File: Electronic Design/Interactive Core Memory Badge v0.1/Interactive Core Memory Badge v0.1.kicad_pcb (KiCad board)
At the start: 2 copper layers, 8 parts, among them Q1 MMBT4403LT1G, Q2 MMBT4401LT1G, U1 Teensy-LC

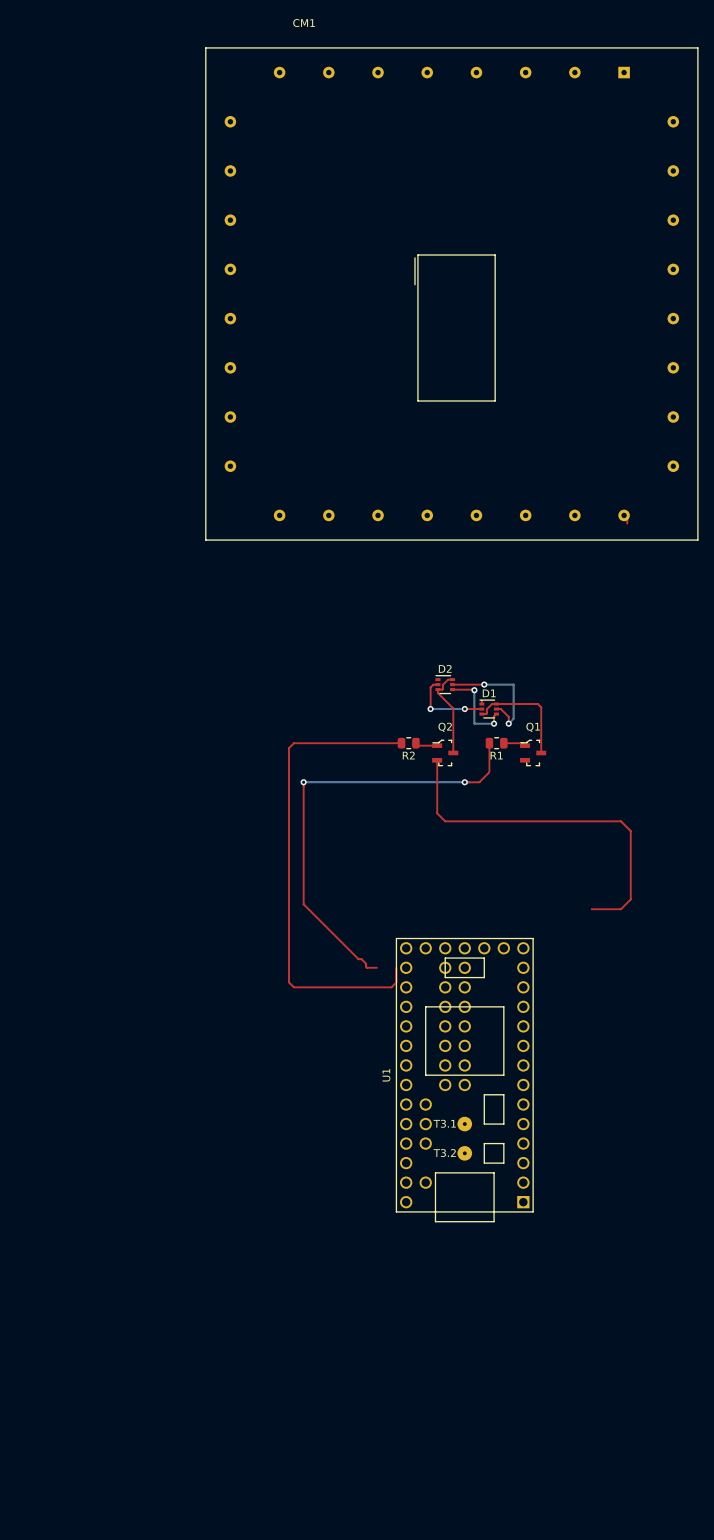
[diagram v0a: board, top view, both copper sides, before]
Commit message: Schematic Complete
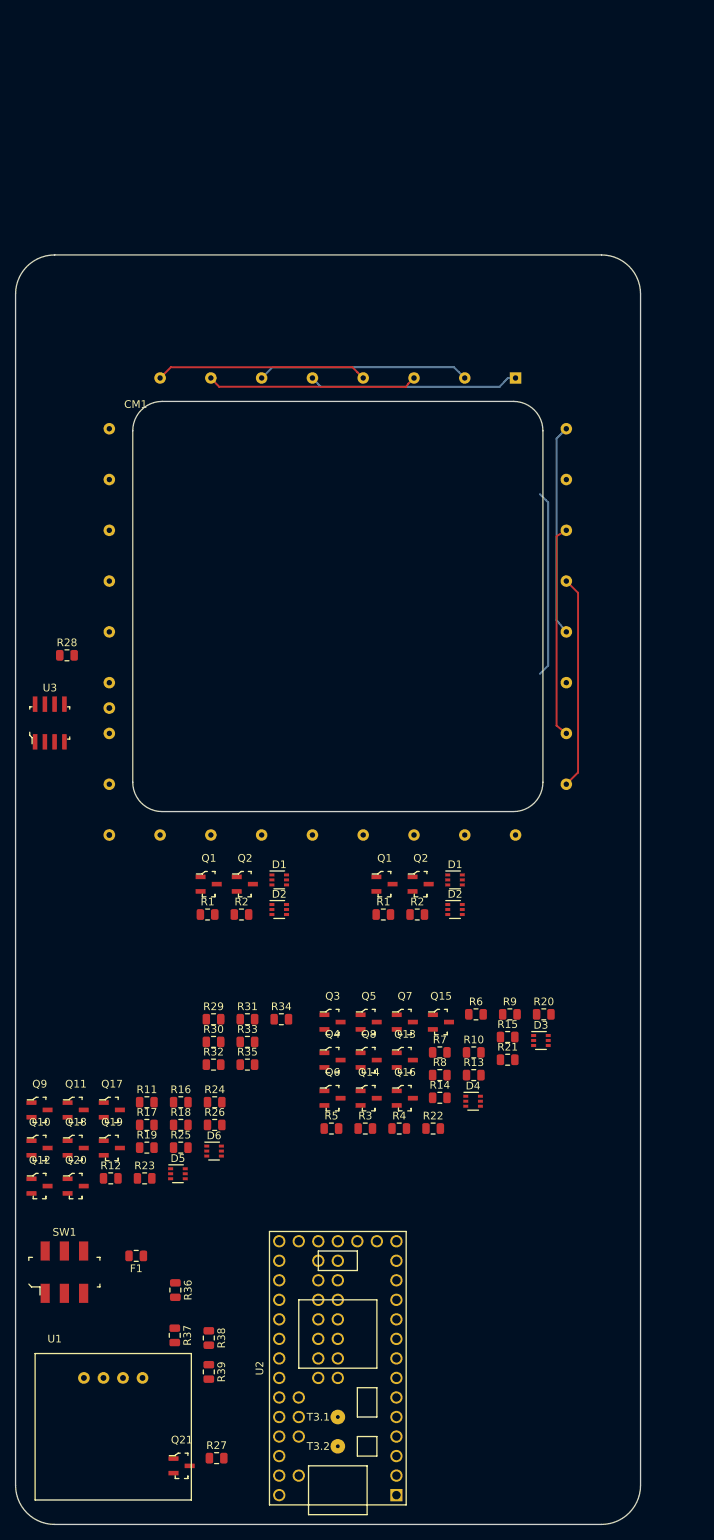
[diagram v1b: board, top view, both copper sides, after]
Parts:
- removed the D1 at (103.5, 89.5)
- removed the D2 at (97.8, 86.4)
- removed the Q1 at (109.2, 95.2)
- removed the Q2 at (97.8, 95.2)
- removed the R1 at (104.5, 94.0)
- removed the R2 at (93.0, 94.0)
- added D1: BAW56S, Package_TO_SOT_SMD:SOT-363_SC-70-6, F.Cu at (99.1, 111.8)
- added D1: BAW56S, Package_TO_SOT_SMD:SOT-363_SC-70-6, F.Cu at (76.2, 111.8)
- added D2: BAV70S, Package_TO_SOT_SMD:SOT-363_SC-70-6, F.Cu at (99.1, 115.6)
- added D2: BAV70S, Package_TO_SOT_SMD:SOT-363_SC-70-6, F.Cu at (76.2, 115.6)
- added D3: BAW56S, Package_TO_SOT_SMD:SOT-363_SC-70-6, F.Cu at (110.2, 132.6)
- added D4: BAV70S, Package_TO_SOT_SMD:SOT-363_SC-70-6, F.Cu at (101.4, 140.5)
- added D5: BAW56S, Package_TO_SOT_SMD:SOT-363_SC-70-6, F.Cu at (63.0, 150.0)
- added D6: BAV70S, Package_TO_SOT_SMD:SOT-363_SC-70-6, F.Cu at (67.7, 147.0)
- added F1: Polyfuse, Fuse:Fuse_0805_2012Metric, F.Cu at (57.6, 160.7)
- added Q1: MMBT4403LT1G, Digikey:SOT-23-3, F.Cu at (89.9, 112.3)
- added Q1: MMBT4403LT1G, Digikey:SOT-23-3, F.Cu at (67.0, 112.3)
- added Q10: MMBT4401LT1G, Digikey:SOT-23-3, F.Cu at (45.0, 146.6)
- added Q11: MMBT4403LT1G, Digikey:SOT-23-3, F.Cu at (49.7, 141.7)
- added Q12: MMBT4401LT1G, Digikey:SOT-23-3, F.Cu at (45.0, 151.6)
- added Q13: MMBT4403LT1G, Digikey:SOT-23-3, F.Cu at (92.5, 135.2)
- added Q14: MMBT4401LT1G, Digikey:SOT-23-3, F.Cu at (87.8, 140.1)
- added Q15: MMBT4403LT1G, Digikey:SOT-23-3, F.Cu at (97.2, 130.2)
- added Q16: MMBT4401LT1G, Digikey:SOT-23-3, F.Cu at (92.5, 140.1)
- added Q17: MMBT4403LT1G, Digikey:SOT-23-3, F.Cu at (54.4, 141.7)
- added Q18: MMBT4401LT1G, Digikey:SOT-23-3, F.Cu at (49.7, 146.6)
- added Q19: MMBT4403LT1G, Digikey:SOT-23-3, F.Cu at (54.4, 146.6)
- added Q2: MMBT4401LT1G, Digikey:SOT-23-3, F.Cu at (94.6, 112.3)
- added Q2: MMBT4401LT1G, Digikey:SOT-23-3, F.Cu at (71.7, 112.3)
- added Q20: MMBT4401LT1G, Digikey:SOT-23-3, F.Cu at (49.7, 151.6)
- added Q21: MMBT4401LT1G, Digikey:SOT-23-3, F.Cu at (63.5, 188.0)
- added Q3: MMBT4403LT1G, Digikey:SOT-23-3, F.Cu at (83.1, 130.2)
- added Q4: MMBT4401LT1G, Digikey:SOT-23-3, F.Cu at (83.1, 135.2)
- added Q5: MMBT4403LT1G, Digikey:SOT-23-3, F.Cu at (87.8, 130.2)
- added Q6: MMBT4401LT1G, Digikey:SOT-23-3, F.Cu at (83.1, 140.1)
- added Q7: MMBT4403LT1G, Digikey:SOT-23-3, F.Cu at (92.5, 130.2)
- added Q8: MMBT4401LT1G, Digikey:SOT-23-3, F.Cu at (87.8, 135.2)
- added Q9: MMBT4403LT1G, Digikey:SOT-23-3, F.Cu at (45.0, 141.7)
- added R1: 220, Resistor_SMD:R_0805_2012Metric, F.Cu at (89.7, 116.3)
- added R1: 220, Resistor_SMD:R_0805_2012Metric, F.Cu at (66.9, 116.3)
- added R10: 6R8, Resistor_SMD:R_0805_2012Metric, F.Cu at (101.5, 134.2)
- added R11: 6R8, Resistor_SMD:R_0805_2012Metric, F.Cu at (59.0, 140.7)
- added R12: 6R8, Resistor_SMD:R_0805_2012Metric, F.Cu at (54.3, 150.6)
- added R13: 220, Resistor_SMD:R_0805_2012Metric, F.Cu at (101.5, 137.1)
- added R14: 220, Resistor_SMD:R_0805_2012Metric, F.Cu at (97.1, 140.1)
- added R15: 6R8, Resistor_SMD:R_0805_2012Metric, F.Cu at (105.9, 132.2)
- added R16: 220, Resistor_SMD:R_0805_2012Metric, F.Cu at (63.4, 140.7)
- added R17: 220, Resistor_SMD:R_0805_2012Metric, F.Cu at (59.0, 143.6)
- added R18: 220, Resistor_SMD:R_0805_2012Metric, F.Cu at (63.4, 143.6)
- added R19: 220, Resistor_SMD:R_0805_2012Metric, F.Cu at (59.0, 146.6)
- added R2: 220, Resistor_SMD:R_0805_2012Metric, F.Cu at (94.2, 116.3)
- added R2: 220, Resistor_SMD:R_0805_2012Metric, F.Cu at (71.3, 116.3)
- added R20: 220, Resistor_SMD:R_0805_2012Metric, F.Cu at (110.6, 129.2)
- added R21: 220, Resistor_SMD:R_0805_2012Metric, F.Cu at (105.9, 135.1)
- added R22: 6R8, Resistor_SMD:R_0805_2012Metric, F.Cu at (96.2, 144.1)
- added R23: 220, Resistor_SMD:R_0805_2012Metric, F.Cu at (58.7, 150.6)
- added R24: 220, Resistor_SMD:R_0805_2012Metric, F.Cu at (67.8, 140.7)
- added R25: 220, Resistor_SMD:R_0805_2012Metric, F.Cu at (63.4, 146.6)
- added R26: 220, Resistor_SMD:R_0805_2012Metric, F.Cu at (67.8, 143.6)
- added R27: 220, Resistor_SMD:R_0805_2012Metric, F.Cu at (68.1, 187.0)
- added R28: 1K5, Resistor_SMD:R_0805_2012Metric, F.Cu at (48.6, 82.5)
- added R29: 1K8, Resistor_SMD:R_0805_2012Metric, F.Cu at (67.7, 129.9)
- added R3: 220, Resistor_SMD:R_0805_2012Metric, F.Cu at (87.4, 144.1)
- added R30: 22, Resistor_SMD:R_0805_2012Metric, F.Cu at (67.7, 132.8)
- added R31: 1K5, Resistor_SMD:R_0805_2012Metric, F.Cu at (72.1, 129.9)
- added R32: 1K8, Resistor_SMD:R_0805_2012Metric, F.Cu at (67.7, 135.8)
- added R33: 22, Resistor_SMD:R_0805_2012Metric, F.Cu at (72.1, 132.8)
- added R34: 1K5, Resistor_SMD:R_0805_2012Metric, F.Cu at (76.5, 129.9)
- added R35: 10k, Resistor_SMD:R_0805_2012Metric, F.Cu at (72.1, 135.8)
- added R36: 10k, Resistor_SMD:R_0805_2012Metric, F.Cu at (62.7, 165.1)
- added R37: 10k, Resistor_SMD:R_0805_2012Metric, F.Cu at (62.6, 171.0)
- added R38: 4K7, Resistor_SMD:R_0805_2012Metric, F.Cu at (67.0, 171.3)
- added R39: 4K7, Resistor_SMD:R_0805_2012Metric, F.Cu at (67.0, 175.7)
- added R4: 220, Resistor_SMD:R_0805_2012Metric, F.Cu at (91.8, 144.1)
- added R5: 6R8, Resistor_SMD:R_0805_2012Metric, F.Cu at (83.0, 144.1)
- added R6: 220, Resistor_SMD:R_0805_2012Metric, F.Cu at (101.8, 129.2)
- added R7: 220, Resistor_SMD:R_0805_2012Metric, F.Cu at (97.1, 134.2)
- added R8: 220, Resistor_SMD:R_0805_2012Metric, F.Cu at (97.1, 137.1)
- added R9: 220, Resistor_SMD:R_0805_2012Metric, F.Cu at (106.2, 129.2)
- added SW1: SW_SPST, Digikey:Switch_Slide_JS202011SCQN, F.Cu at (48.3, 162.8)
- added U1: Micro_LiPo_Charger, Core_Memory_8x8_Array:Micro_LiPo_Charger, F.Cu at (54.6, 182.9)
- added U3: LM393, Digikey:SOIC-8_W3.9mm, F.Cu at (46.4, 91.3)
- moved CM1 43.3 mm to (83.8, 76.2)
- moved U2 41.5 mm to (83.8, 175.3)
- renumbered U1 to U2
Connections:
- net Net-(U1-Pad19) renamed AVAILABLE
- net Net-(U1-Pad37) renamed REED_SWITCH
- CM1 pad 1: XT0 -> XT0-4
- CM1 pad 10: Net-(CM1-Pad10) -> YL1
- CM1 pad 11: Net-(CM1-Pad11) -> YL2
- CM1 pad 12: Net-(CM1-Pad12) -> YL3
- CM1 pad 13: Net-(CM1-Pad13) -> YL4
- CM1 pad 14: Net-(CM1-Pad10) -> YL5
- CM1 pad 15: Net-(CM1-Pad11) -> YL4
- CM1 pad 16: Net-(CM1-Pad12) -> YL5
- CM1 pad 2: XT1 -> XT1-5
- CM1 pad 29: Net-(CM1-Pad29) -> Net-(CM1-Pad25)
- CM1 pad 3: XT2 -> XT2-6
- CM1 pad 30: Net-(CM1-Pad30) -> Net-(CM1-Pad26)
- CM1 pad 31: Net-(CM1-Pad31) -> Net-(CM1-Pad27)
- CM1 pad 32: Net-(CM1-Pad32) -> Net-(CM1-Pad28)
- CM1 pad 4: XT3 -> XT3-7
- CM1 pad 5: XT4 -> XT0-4
- CM1 pad 6: XT5 -> XT1-5
- CM1 pad 7: XT6 -> XT2-6
- CM1 pad 8: XT7 -> XT3-7
- CM1 pad 9: Net-(CM1-Pad13) -> YL0
- U2 pad 1: Net-(U1-Pad1) -> -BATT
- U2 pad 10: Net-(U1-Pad10) -> Q4N
- U2 pad 11: Net-(U1-Pad11) -> Q5P
- U2 pad 12: Net-(U1-Pad12) -> Q5N
- U2 pad 13: Net-(U1-Pad13) -> Q6P
- U2 pad 14: Net-(U1-Pad14) -> Q6N
- U2 pad 2: Net-(U1-Pad2) -> SENSE_PULSE
- U2 pad 20: Net-(U1-Pad20) -> Q7P
- U2 pad 21: Net-(U1-Pad21) -> Q7N
- U2 pad 22: Net-(U1-Pad22) -> Q8P
- U2 pad 23: Net-(U1-Pad23) -> Q8N
- U2 pad 24: Net-(U1-Pad24) -> Q9P
- U2 pad 25: Net-(U1-Pad25) -> I2C_DATA
- U2 pad 26: Net-(U1-Pad26) -> I2C_CLOCK
- U2 pad 27: Net-(U1-Pad27) -> Q9N
- U2 pad 28: Net-(U1-Pad28) -> Q10P
- U2 pad 29: Net-(U1-Pad29) -> Q10N
- U2 pad 30: Net-(U1-Pad30) -> WRITE_ENABLE
- U2 pad 31: Net-(U1-Pad31) -> +3V3
- U2 pad 32: Net-(U1-Pad32) -> -BATT
- U2 pad 33: +BATT -> +VSW
- U2 pad 34: Net-(U1-Pad34) -> V+USB
- U2 pad 35: Net-(U1-Pad35) -> +3V3
- U2 pad 5: Net-(U1-Pad5) -> Q2P
- U2 pad 6: Net-(U1-Pad6) -> Q2N
- U2 pad 7: Net-(U1-Pad7) -> Q3P
- U2 pad 8: Net-(U1-Pad8) -> Q3N
- U2 pad 9: Net-(U1-Pad9) -> Q4P
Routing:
- net Q1N: track 61.8 -> 0.00 mm
- net Q1P: track 57.9 -> 0.00 mm, vias 2 -> 0
- net -BATT: track 47.5 -> 0.00 mm
- net Net-(CM1-Pad26): track 0.00 -> 27.7 mm
- net Net-(CM1-Pad25): track 0.00 -> 27.7 mm
- net XT3-7: track 0.00 -> 27.6 mm
- net XT1-5: track 0.00 -> 27.6 mm
- net XT2-6: track 0.00 -> 27.4 mm
- net XT0-4: track 0.00 -> 27.4 mm
- net Net-(CM1-Pad28): track 0.00 -> 27.4 mm
- net Net-(CM1-Pad27): track 0.00 -> 24.3 mm
- net XB4: track 16.2 -> 0.00 mm, vias 2 -> 0
- net Net-(D1-Pad3): track 14.7 -> 0.00 mm
- net Net-(D2-Pad3): track 11.8 -> 0.00 mm
- net XB5: track 11.2 -> 0.00 mm, vias 2 -> 0
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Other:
- board outline added: 81.3 x 165.1 mm
